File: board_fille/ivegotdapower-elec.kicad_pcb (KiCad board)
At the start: 2 copper layers, 45 x 23 mm, 16 parts, among them J1 Conn_02x03_Odd_Even, J2 Conn_02x03_Odd_Even, U1 LM2596S-ADJ

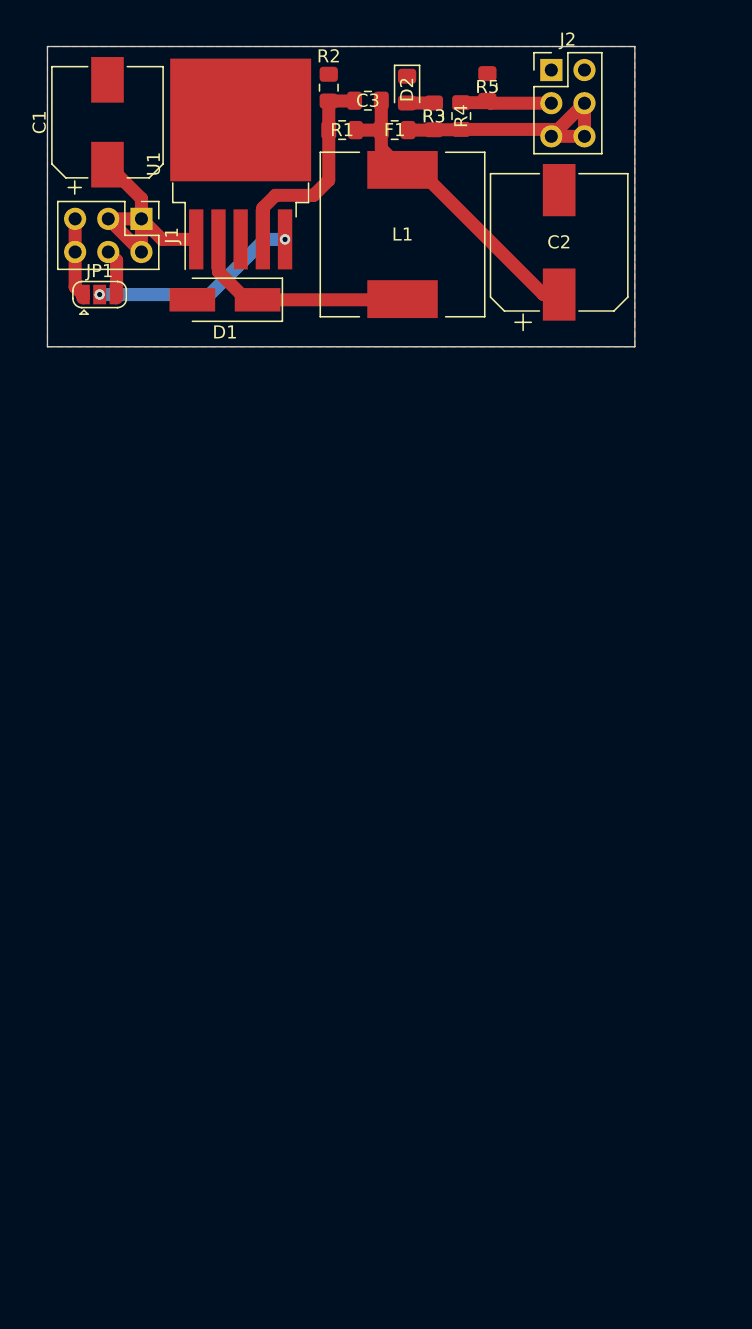
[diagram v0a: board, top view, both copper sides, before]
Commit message: cleanup, finished design
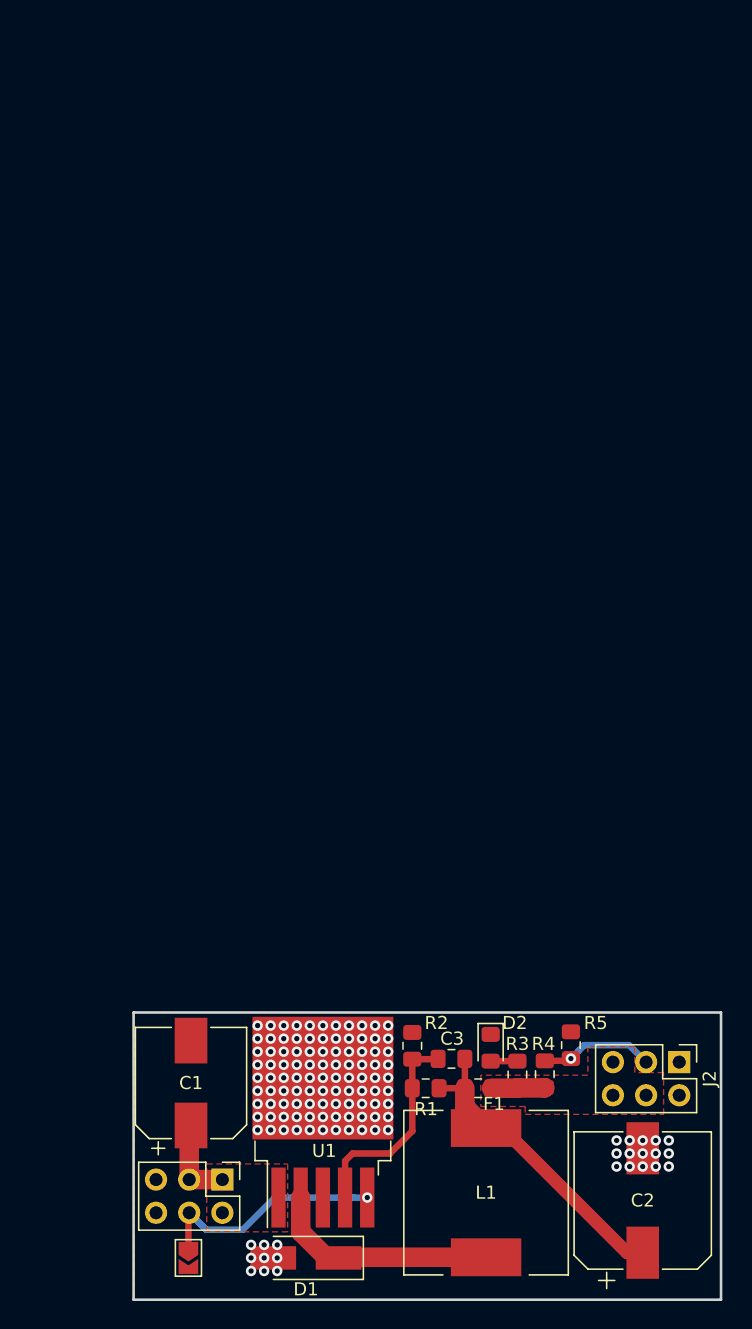
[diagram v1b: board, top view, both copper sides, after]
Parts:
- JP1: value Jumper_NC_Dual -> SolderJumper_2_Open; footprint Jumper:SolderJumper-3_P1.3mm_Open_RoundedPad1.0x1.5mm -> Jumper:SolderJumper-2_P1.3mm_Open_TrianglePad1.0x1.5mm
- moved J2 76.6 mm to (141.8, 103.8), turned to 270 degrees
- moved JP1 74.1 mm to (104.2, 118.8), turned to 270 degrees
- moved C1 73.9 mm to (104.4, 105.4)
- moved J1 73.9 mm to (106.8, 112.8)
- moved C2 73.7 mm to (139.0, 114.4)
- moved C3 73.7 mm to (124.3, 103.5)
- moved D2 73.7 mm to (127.3, 102.7)
- moved F1 73.7 mm to (126.4, 105.8)
- moved L1 73.7 mm to (127.0, 113.8)
- moved R1 73.7 mm to (122.4, 105.8)
- moved R2 73.7 mm to (121.3, 102.5)
- moved R3 73.7 mm to (129.4, 104.8)
- moved R5 73.7 mm to (133.5, 102.5)
- moved R4 73.7 mm to (131.5, 104.7)
- moved U1 73.7 mm to (114.5, 108.4)
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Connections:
- JP1 pad 1: GND -> /on-off
- JP1 pad 2: Net-(JP1-Pad2) -> GND
- U1 pad 5: Net-(JP1-Pad2) -> /on-off
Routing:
- net /on-off: track 3.53 -> 19.8 mm, vias 0 -> 1
- net /Power_Output: track 20.2 -> 4.10 mm
- net Net-(JP1-Pad2): track 16.0 -> 0.00 mm, vias 2 -> 0
- net /Power_Input: track 18.8 -> 6.75 mm
- net GND: track 6.04 -> 0.00 mm, vias 0 -> 123
- net /voltage_measure: track 7.06 -> 8.80 mm, vias 0 -> 1
- added copper zone on F.Cu, net /Power_Input
- added copper zone on F.Cu, net /Power_Output
- added copper zone on B.Cu, net GND
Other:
- board size 45 x 23 mm -> 45 x 22 mm

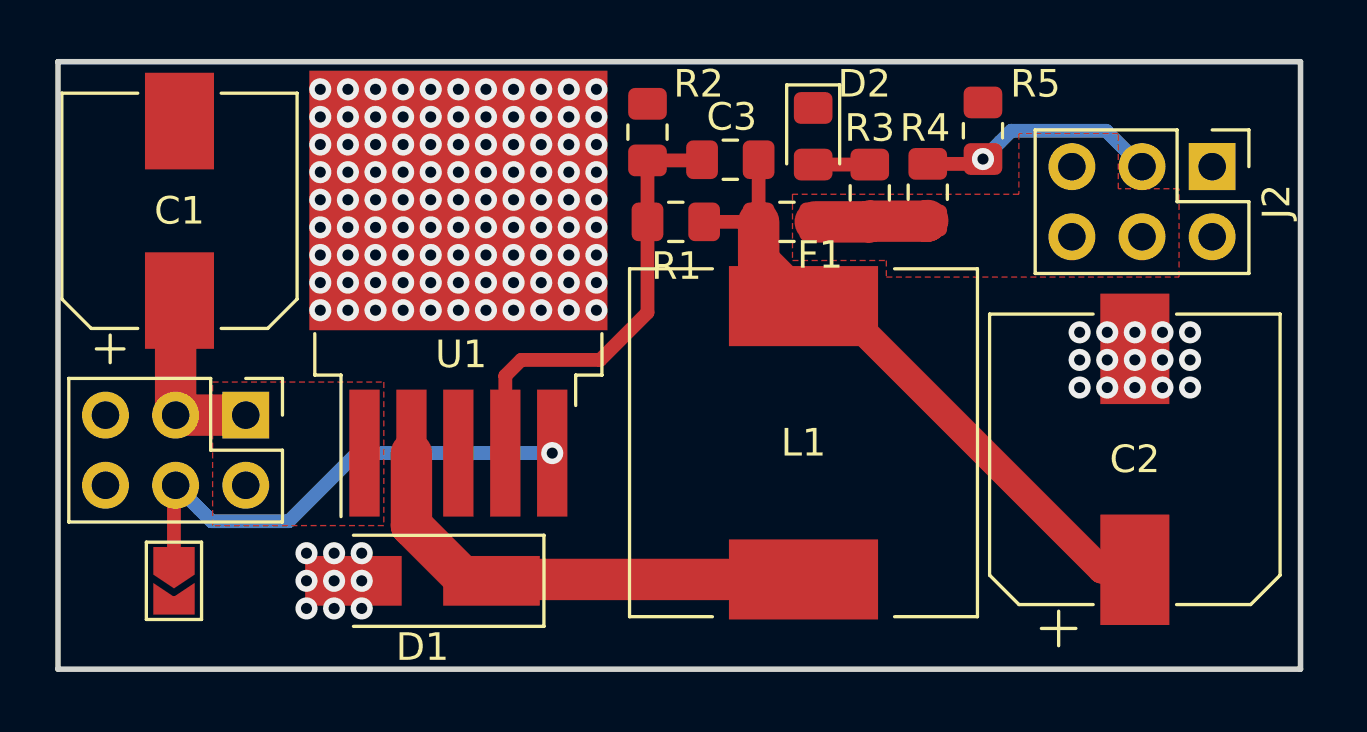
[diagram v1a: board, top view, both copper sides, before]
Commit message: very small changes in fille
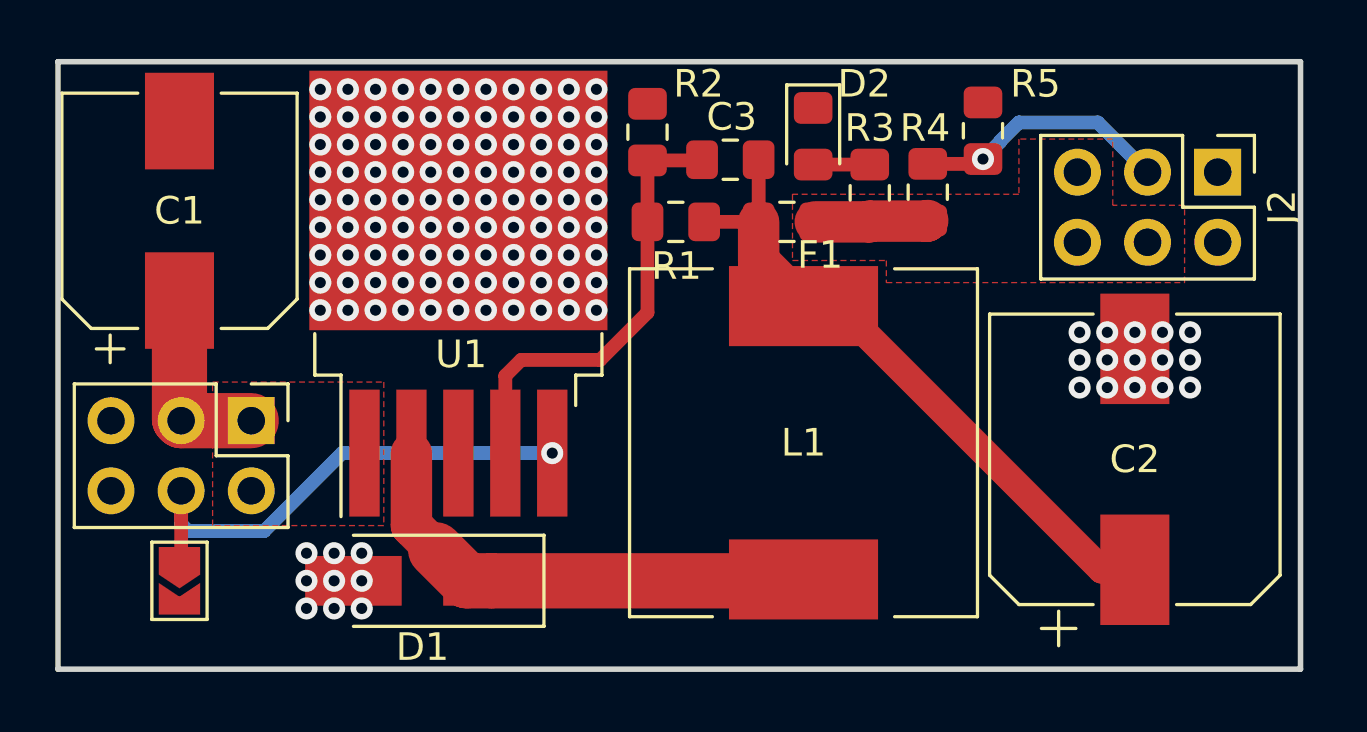
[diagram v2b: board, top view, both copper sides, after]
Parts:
- moved J1 0.28 mm to (107.0, 113.0)
- moved J2 0.28 mm to (142.0, 104.0)
- moved JP1 0.20 mm to (104.4, 118.8)
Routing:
- net /on-off: track 19.8 -> 18.5 mm
